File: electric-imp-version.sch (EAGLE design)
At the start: 42 parts, among them Q1 DMG2307L-7, U1 ELECTRIC_IMP, U2 TPS62172, U3 ATSHA204-TSU, U4 MCP73831, U5 CD74HC4067-SSOPCD74HC4067, U6 CD74HC4067-SSOPCD74HC4067, U7 LTC6904LTC6904, X1 USBSMD

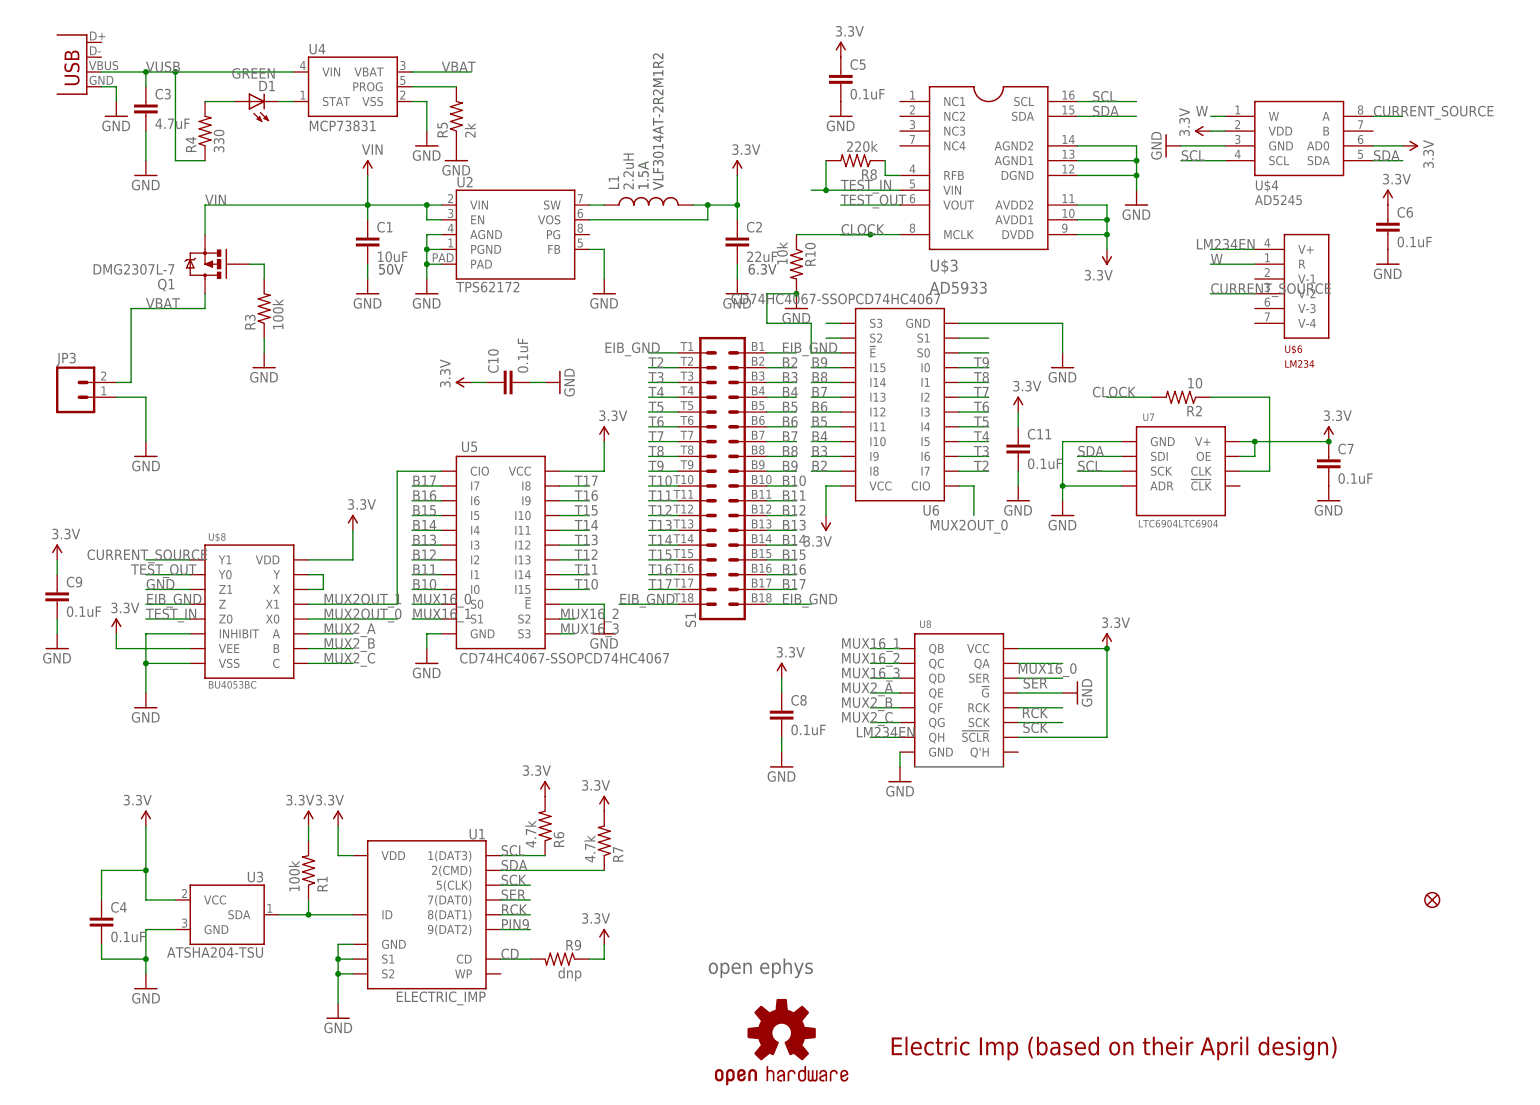
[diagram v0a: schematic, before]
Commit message: Aesthetic fixes
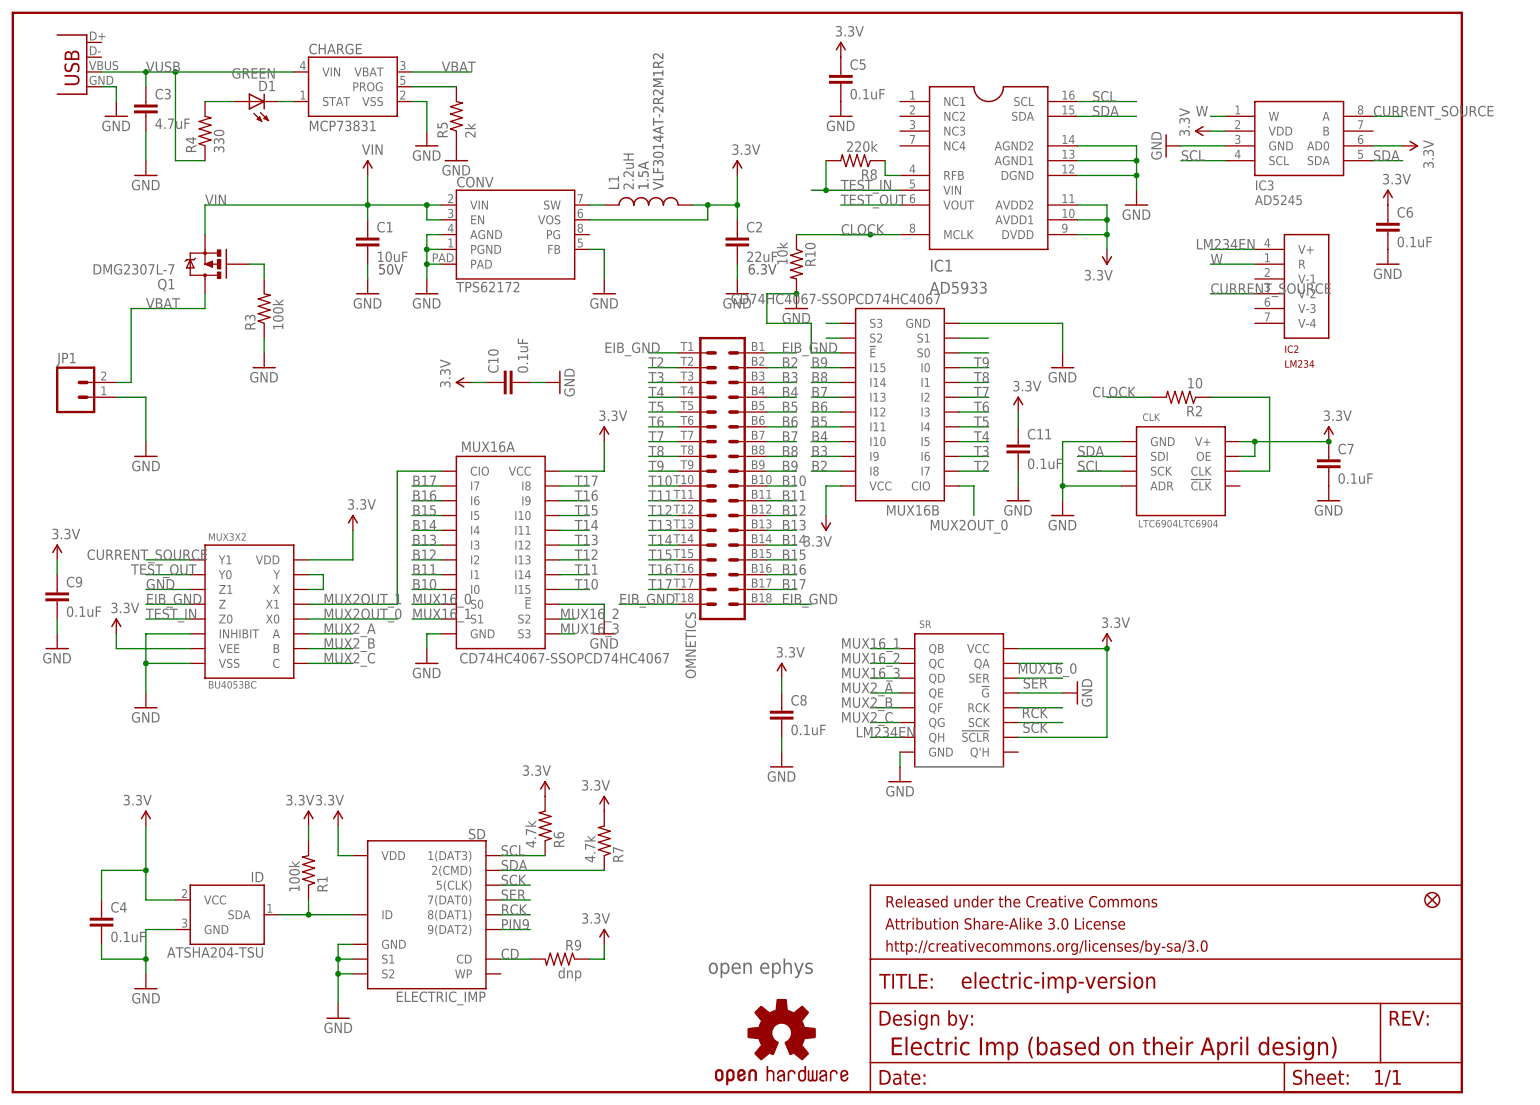
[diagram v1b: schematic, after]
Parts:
- added FRAME1: FRAME-LETTER, SparkFun-Aesthetics:FRAME-LETTER
- renumbered JP3 to JP1, S1 to OMNETICS, U$3 to IC1, U$4 to IC3, U$6 to IC2, U$8 to MUX3X2, U1 to SD, U2 to CONV, U3 to ID, U4 to CHARGE, U5 to MUX16A, U6 to MUX16B, U7 to CLK, U8 to SR, X1 to USB
